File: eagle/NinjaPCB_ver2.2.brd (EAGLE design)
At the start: 79 x 73 mm, 72 parts, among them IC1 ANALOGSW_AD_SOT23-6, IC2 NAU7802, Q1 IRLB3813PBF, Q2 CJ2302, Q3 CJ2302, Q4 S9013, Q5 S9013, Q6 S9013

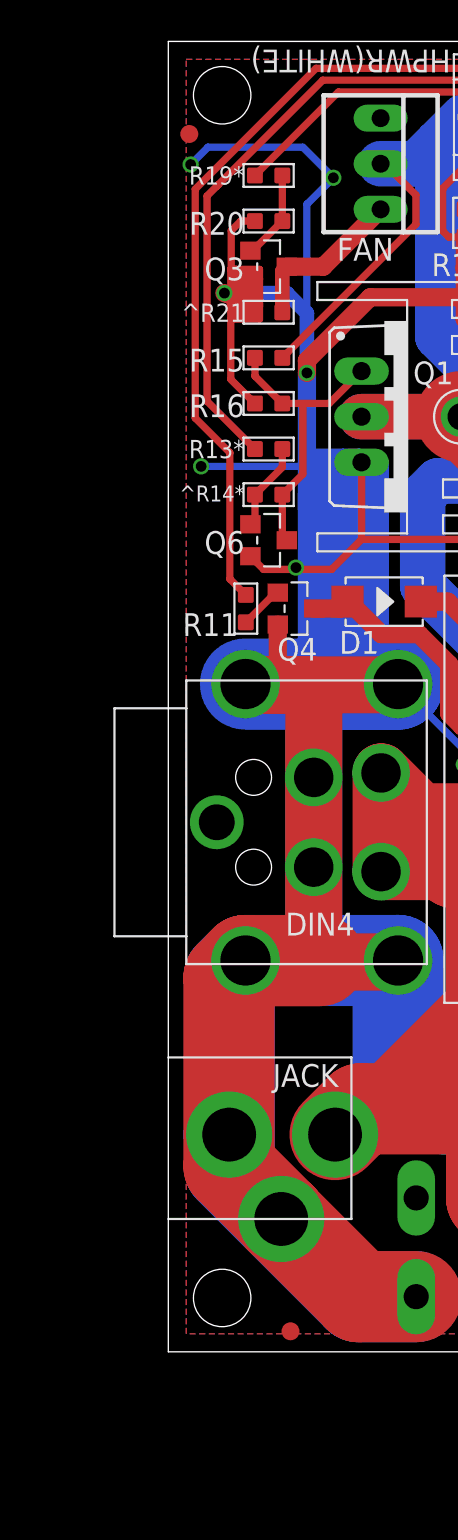
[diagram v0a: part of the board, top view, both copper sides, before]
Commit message: sync
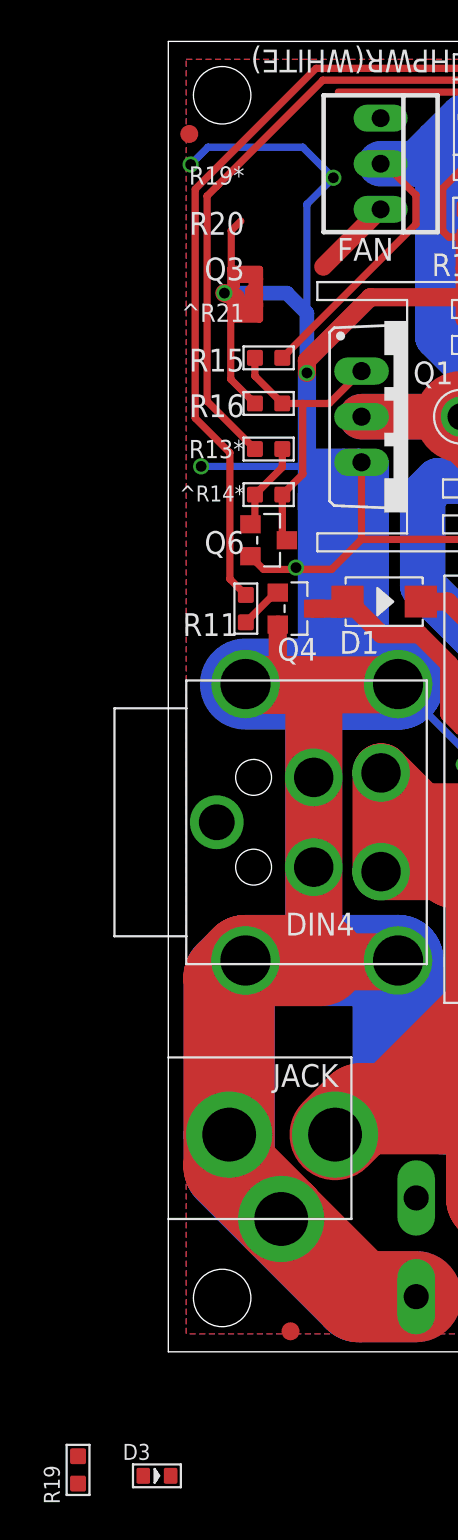
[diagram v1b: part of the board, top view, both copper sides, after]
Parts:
- removed Q3: CJ2302, Seeed-Transistor:SOT-23
- removed R20: 10K 1/10W, Seeed-Resistor:R0603
- removed R21: 0R, Seeed-Resistor:R0603
- added D3: YELLOW-0603, Seeed-LED:LED-0603
- R14: value 1K 1/10W -> 0R
- moved R19 72.9 mm to (-5.03, -6.58), turned to 0 degrees
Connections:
- net MODE renamed TOUT
- removed net FAN: ESP1.18, ESP2.P$8, ESP3.P$8, IO0.1, R19.1, R2.2
- removed net N$8: Q3.1, R19.2, R20.2
- new net IO0: D3.+, ESP1.18, ESP2.P$8, ESP3.P$8, IO0.1, R2.2
- net GND: now also FAN.3, R19.1; no longer Q3.2, R20.1, R21.1
- net N$4: now also D3.-, R19.2; no longer FAN.3, Q3.3, R21.2
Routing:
- net FAN: track 165.0 -> 0.00 mm, vias 3 -> 0
- net IO0: track 0.00 -> 158.4 mm, vias 0 -> 3
- net N$4: track 9.19 -> 0.00 mm
- net N$8: track 5.00 -> 0.00 mm
- net GND: track 878.0 -> 879.6 mm
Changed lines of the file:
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@@
 <attribute name="MPN" value="RC0603JR-0710KL" x="138.176" y="130.1496" size="1.778" layer="27" rot="R90" display="off"/>
-</element>
-<element name="R19" library="Seeed-Resistor" package="R0603" value="1K 1/10W" x="5.588" y="65.532" smashed="yes" rot="R90">
-<attribute name="MPN" value="RC0603JR-071KL" x="102.108" y="146.812" size="1.778" layer="27" rot="R90" display="off"/>
 </element>
 <element name="R17" library="Seeed-Resistor" package="R0603" value="1K 1/10W" x="19.05" y="62.8904" smashed="yes">
@@
 <element name="R18" library="Seeed-Resistor" package="R0603" value="10K 1/10W" x="16.51" y="62.8904" smashed="yes" rot="R180">
 <attribute name="MPN" value="RC0603JR-0710KL" x="-34.29" y="159.4104" size="1.778" layer="27" rot="R180" display="off"/>
-</element>
-<element name="R20" library="Seeed-Resistor" package="R0603" value="10K 1/10W" x="5.588" y="62.992" smashed="yes" rot="R90">
-<attribute name="MPN" value="RC0603JR-0710KL" x="102.108" y="118.872" size="1.778" layer="27" rot="R90" display="off"/>
 </element>
 <element name="R13" library="Seeed-Resistor" package="R0603" value="1K 1/10W" x="5.588" y="50.292" smashed="yes" rot="R90">
@@
 <element name="Q2" library="Seeed-Transistor" package="SOT-23" value="CJ2302" x="26.0434" y="59.635" smashed="yes" rot="R270">
 <attribute name="MPN" value="CJ2302" x="-55.2366" y="-1.325" size="1.778" layer="27" rot="R270" display="off"/>
-</element>
-<element name="Q3" library="Seeed-Transistor" package="SOT-23" value="CJ2302" x="5.588" y="60.452" smashed="yes" rot="R270">
-<attribute name="MPN" value="CJ2302" x="-75.692" y="-5.588" size="1.778" layer="27" rot="R270" display="off"/>
 </element>
 <element name="SERIAL6" library="pinhead" package="1X06" value="" x="45.0342" y="13.1826" smashed="yes" rot="MR0">
@@
 <element name="U$9" library="adafruit" package="FIDUCIAL_1MM" value="FIDUCIAL" x="53.467" y="46.609" smashed="yes" rot="R270"/>
 <element name="U$10" library="adafruit" package="FIDUCIAL_1MM" value="FIDUCIAL" x="77.851" y="40.513" smashed="yes" rot="R270"/>
-<element name="R14" library="Seeed-Resistor" package="R0603" value="1K 1/10W" x="5.588" y="47.752" smashed="yes" rot="R90">
-<attribute name="MPN" value="RC0603JR-071KL" x="102.108" y="134.112" size="1.778" layer="27" rot="R90" display="off"/>
-</element>
-<element name="R21" library="Seeed-Resistor" package="R0603" value="0R" x="5.588" y="57.912" smashed="yes" rot="R90">
-<attribute name="MPN" value="RC0603JR-070RL" x="108.458" y="117.602" size="1.778" layer="27" rot="R90" display="off"/>
+<element name="R14" library="Seeed-Resistor" package="R0603" value="0R" x="5.588" y="47.752" smashed="yes" rot="R90">
+<attribute name="MPN" value="RC0603JR-070RL" x="102.108" y="134.112" size="1.778" layer="27" rot="R90" display="off"/>
 </element>
 <element name="PELTIER" library="Seeed-Connector" package="H2-3.5-7.0X7.0MM" value="" x="35.775" y="34.9708" smashed="yes">
@@
 <element name="U$1" library="oshw" package="OSHW_5MM" value="" x="68.834" y="69.5198"/>
 <element name="U$2" library="oshw" package="OSHW_5MM" value="" x="75.3872" y="64.5922" rot="MR0"/>
+<element name="D3" library="Seeed-LED" package="LED-0603" value="YELLOW-0603" x="-0.635" y="-6.9088">
+<attribute name="MPN" value="19-217-Y5C-AM1N1VY-3T" x="-0.635" y="-6.9088" size="1.778" layer="27" display="off"/>
+</element>
+<element name="R19" library="Seeed-Resistor" package="R0603" value="1K 1/10W" x="-5.0292" y="-6.5786">
+<attribute name="MPN" value="RC0603JR-071KL" x="-5.0292" y="-6.5786" size="1.778" layer="27" display="off"/>
+</element>
 </elements>
 <signals>
@@
 <contactref element="Q2" pad="2"/>
 <contactref element="R18" pad="1"/>
-<contactref element="Q3" pad="2"/>
-<contactref element="R20" pad="1"/>
-<contactref element="R21" pad="1"/>
 <contactref element="SERIAL6" pad="6"/>
 <contactref element="ESP3" pad="P$9"/>
@@
 <wire x1="9.0932" y1="43.5864" x2="10.7638" y2="45.257" width="0.4064" layer="1"/>
 <wire x1="10.7638" y1="45.257" x2="10.7638" y2="49.5542" width="0.4064" layer="1"/>
-<wire x1="4.826" y1="59.309" x2="4.572" y2="59.563" width="0.4064" layer="1"/>
-<wire x1="4.826" y1="62.992" x2="4.0386" y2="62.992" width="0.4064" layer="1"/>
 <via x="3.1242" y="58.9788" extent="1-16" drill="0.6" shape="square"/>
 <wire x1="3.1242" y1="58.9788" x2="3.7592" y2="58.7502" width="1.016" layer="1"/>
-<wire x1="3.7592" y1="58.7502" x2="4.572" y2="59.563" width="1.016" layer="1"/>
-<wire x1="4.2926" y1="59.563" x2="4.572" y2="59.563" width="0.4064" layer="1"/>
 <wire x1="4.7752" y1="57.8866" x2="3.9624" y2="57.8866" width="0.8128" layer="1"/>
 <wire x1="3.9624" y1="57.8866" x2="3.6576" y2="58.1914" width="0.8128" layer="1"/>
@@
 <wire x1="3.5052" y1="60.325" x2="4.064" y2="59.7662" width="0.4064" layer="1"/>
 <wire x1="4.064" y1="59.7662" x2="4.3688" y2="59.7662" width="0.4064" layer="1"/>
-<wire x1="4.3688" y1="59.7662" x2="4.572" y2="59.563" width="0.4064" layer="1"/>
-<wire x1="4.826" y1="57.912" x2="4.8006" y2="57.912" width="0.4064" layer="1"/>
 <wire x1="4.8006" y1="57.912" x2="4.7752" y2="57.8866" width="0.4064" layer="1"/>
 <wire x1="8.4836" y1="49.2252" x2="10.4348" y2="49.2252" width="1.016" layer="16"/>
@@
 <wire x1="51.3588" y1="53.6702" x2="50.5206" y2="52.832" width="0.4064" layer="1"/>
 <wire x1="50.5206" y1="52.832" x2="48.768" y2="52.832" width="0.4064" layer="1"/>
+<contactref element="FAN" pad="3"/>
+<wire x1="11.8274" y1="63.6456" x2="8.6338" y2="60.452" width="1.016" layer="1"/>
+<contactref element="R19" pad="1"/>
+<wire x1="56.7436" y1="25.2984" x2="51.7398" y2="29.4386" width="0" layer="19" extent="1-1"/>
+<wire x1="5.08" y1="59.7408" x2="4.8768" y2="59.817" width="0" layer="19" extent="1-1"/>
+<wire x1="8.6338" y1="60.452" x2="6.604" y2="58.9788" width="0" layer="19" extent="1-16"/>
+<wire x1="71.7804" y1="3.2004" x2="77.159" y2="6.817" width="0" layer="19" extent="1-1"/>
+<wire x1="61.7982" y1="5.8674" x2="67.6656" y2="11.1252" width="0" layer="19" extent="1-1"/>
+<wire x1="-5.0292" y1="-5.8166" x2="6.29" y2="7.4" width="0" layer="19" extent="1-1"/>
 </signal>
 <signal name="3V3">
@@
 <wire x1="32.893" y1="47.4472" x2="33.0454" y2="47.4472" width="0.4064" layer="16"/>
 </signal>
-<signal name="N$4">
-<contactref element="FAN" pad="3"/>
-<contactref element="Q3" pad="3"/>
-<contactref element="R21" pad="2"/>
-<wire x1="11.8274" y1="63.6456" x2="8.6338" y2="60.452" width="1.016" layer="1"/>
-<wire x1="8.6338" y1="60.452" x2="6.604" y2="60.452" width="1.016" layer="1"/>
-<wire x1="6.35" y1="57.912" x2="6.35" y2="60.198" width="0.8128" layer="1"/>
-<wire x1="6.35" y1="60.198" x2="6.604" y2="60.452" width="0.8128" layer="1"/>
-</signal>
-<signal name="FAN">
-<contactref element="R19" pad="1"/>
+<signal name="IO0">
 <contactref element="ESP2" pad="P$8"/>
 <contactref element="ESP1" pad="18"/>
@@
 <contactref element="ESP3" pad="P$8"/>
 <contactref element="IO0" pad="1"/>
-<wire x1="4.826" y1="65.532" x2="9.4742" y2="70.1802" width="0.4064" layer="1"/>
 <wire x1="58.1844" y1="43.239" x2="58.1844" y2="41.6884" width="0.4064" layer="1"/>
 <wire x1="58.1844" y1="41.6884" x2="58.9026" y2="40.9702" width="0.4064" layer="1"/>
@@
 <wire x1="60.7568" y1="52.9336" x2="59.1312" y2="54.5592" width="0.4064" layer="1"/>
 <wire x1="59.1312" y1="54.5592" x2="59.1312" y2="59.5884" width="0.4064" layer="1"/>
+<contactref element="D3" pad="+"/>
+<wire x1="-1.397" y1="-6.9088" x2="42.4942" y2="11.6586" width="0" layer="19" extent="1-1"/>
 </signal>
 <signal name="PEL_PWM">
@@
 <wire x1="32.512" y1="61.976" x2="32.512" y2="62.992" width="0.4064" layer="1"/>
 </signal>
-<signal name="MODE">
+<signal name="TOUT">
 <contactref element="ESP1" pad="2"/>
 <contactref element="ESP2" pad="P$16"/>
@@
 <wire x1="65.405" y1="58.166" x2="65.7352" y2="57.8358" width="0.4064" layer="16"/>
 </signal>
-<signal name="N$8">
+<signal name="N$4">
+<contactref element="D3" pad="-"/>
 <contactref element="R19" pad="2"/>
-<contactref element="Q3" pad="1"/>
-<contactref element="R20" pad="2"/>
-<wire x1="4.572" y1="61.341" x2="4.699" y2="61.341" width="0.4064" layer="1"/>
-<wire x1="4.699" y1="61.341" x2="6.35" y2="62.992" width="0.4064" layer="1"/>
-<wire x1="6.35" y1="65.532" x2="6.35" y2="62.992" width="0.4064" layer="1"/>
+<wire x1="0.127" y1="-6.9088" x2="-5.0292" y2="-7.3406" width="0" layer="19" extent="1-1"/>
 </signal>
 </signals>

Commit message: add NinjaPCR 2.2
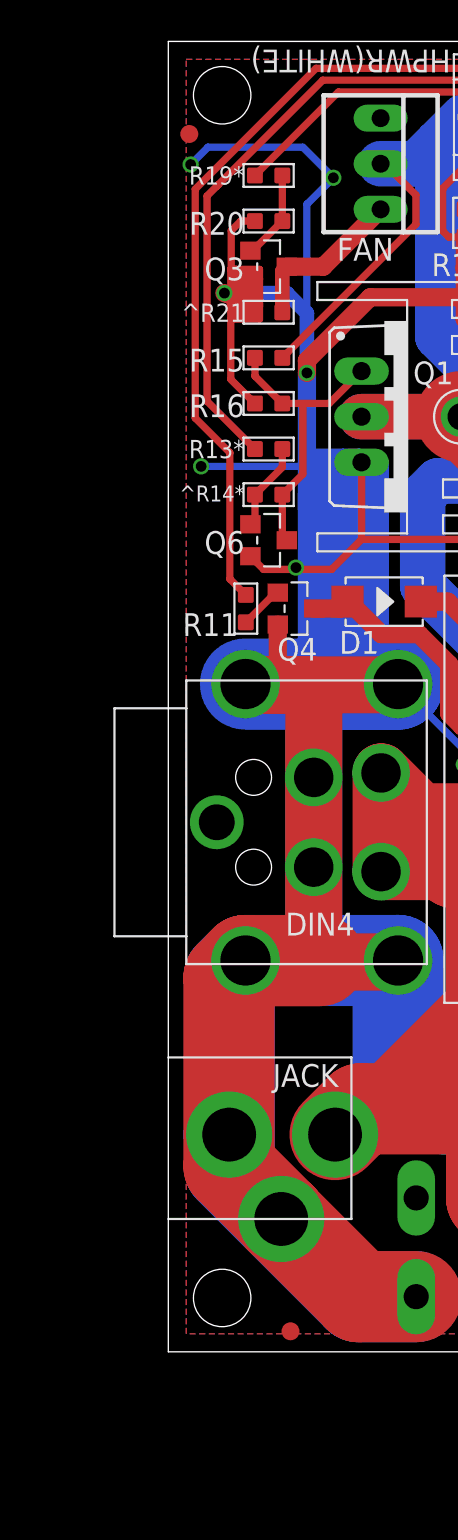
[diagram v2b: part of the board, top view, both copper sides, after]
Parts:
- removed D3: YELLOW-0603, Seeed-LED:LED-0603
- added Q3: CJ2302, Seeed-Transistor:SOT-23
- added R20: 10K 1/10W, Seeed-Resistor:R0603
- added R21: 0R, Seeed-Resistor:R0603
- R14: value 0R -> 1K 1/10W
- moved R19 72.9 mm to (5.59, 65.5), turned to 90 degrees
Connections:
- net TOUT renamed MODE
- removed net IO0: D3.+, ESP1.18, ESP2.P$8, ESP3.P$8, IO0.1, R2.2
- new net FAN: ESP1.18, ESP2.P$8, ESP3.P$8, IO0.1, R19.1, R2.2
- new net N$8: Q3.1, R19.2, R20.2
- net GND: now also Q3.2, R20.1, R21.1; no longer FAN.3, R19.1
- net N$4: now also FAN.3, Q3.3, R21.2; no longer D3.-, R19.2
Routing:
- net FAN: track 0.00 -> 165.0 mm, vias 0 -> 3
- net IO0: track 158.4 -> 0.00 mm, vias 3 -> 0
- net N$4: track 0.00 -> 9.19 mm
- net N$8: track 0.00 -> 5.00 mm
- net GND: track 879.6 -> 878.0 mm
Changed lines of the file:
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@@
 <attribute name="MPN" value="RC0603JR-0710KL" x="138.176" y="130.1496" size="1.778" layer="27" rot="R90" display="off"/>
+</element>
+<element name="R19" library="Seeed-Resistor" package="R0603" value="1K 1/10W" x="5.588" y="65.532" smashed="yes" rot="R90">
+<attribute name="MPN" value="RC0603JR-071KL" x="102.108" y="146.812" size="1.778" layer="27" rot="R90" display="off"/>
 </element>
 <element name="R17" library="Seeed-Resistor" package="R0603" value="1K 1/10W" x="19.05" y="62.8904" smashed="yes">
@@
 <element name="R18" library="Seeed-Resistor" package="R0603" value="10K 1/10W" x="16.51" y="62.8904" smashed="yes" rot="R180">
 <attribute name="MPN" value="RC0603JR-0710KL" x="-34.29" y="159.4104" size="1.778" layer="27" rot="R180" display="off"/>
+</element>
+<element name="R20" library="Seeed-Resistor" package="R0603" value="10K 1/10W" x="5.588" y="62.992" smashed="yes" rot="R90">
+<attribute name="MPN" value="RC0603JR-0710KL" x="102.108" y="118.872" size="1.778" layer="27" rot="R90" display="off"/>
 </element>
 <element name="R13" library="Seeed-Resistor" package="R0603" value="1K 1/10W" x="5.588" y="50.292" smashed="yes" rot="R90">
@@
 <element name="Q2" library="Seeed-Transistor" package="SOT-23" value="CJ2302" x="26.0434" y="59.635" smashed="yes" rot="R270">
 <attribute name="MPN" value="CJ2302" x="-55.2366" y="-1.325" size="1.778" layer="27" rot="R270" display="off"/>
+</element>
+<element name="Q3" library="Seeed-Transistor" package="SOT-23" value="CJ2302" x="5.588" y="60.452" smashed="yes" rot="R270">
+<attribute name="MPN" value="CJ2302" x="-75.692" y="-5.588" size="1.778" layer="27" rot="R270" display="off"/>
 </element>
 <element name="SERIAL6" library="pinhead" package="1X06" value="" x="45.0342" y="13.1826" smashed="yes" rot="MR0">
@@
 <element name="U$9" library="adafruit" package="FIDUCIAL_1MM" value="FIDUCIAL" x="53.467" y="46.609" smashed="yes" rot="R270"/>
 <element name="U$10" library="adafruit" package="FIDUCIAL_1MM" value="FIDUCIAL" x="77.851" y="40.513" smashed="yes" rot="R270"/>
-<element name="R14" library="Seeed-Resistor" package="R0603" value="0R" x="5.588" y="47.752" smashed="yes" rot="R90">
-<attribute name="MPN" value="RC0603JR-070RL" x="102.108" y="134.112" size="1.778" layer="27" rot="R90" display="off"/>
+<element name="R14" library="Seeed-Resistor" package="R0603" value="1K 1/10W" x="5.588" y="47.752" smashed="yes" rot="R90">
+<attribute name="MPN" value="RC0603JR-071KL" x="102.108" y="134.112" size="1.778" layer="27" rot="R90" display="off"/>
+</element>
+<element name="R21" library="Seeed-Resistor" package="R0603" value="0R" x="5.588" y="57.912" smashed="yes" rot="R90">
+<attribute name="MPN" value="RC0603JR-070RL" x="108.458" y="117.602" size="1.778" layer="27" rot="R90" display="off"/>
 </element>
 <element name="PELTIER" library="Seeed-Connector" package="H2-3.5-7.0X7.0MM" value="" x="35.775" y="34.9708" smashed="yes">
@@
 <element name="U$1" library="oshw" package="OSHW_5MM" value="" x="68.834" y="69.5198"/>
 <element name="U$2" library="oshw" package="OSHW_5MM" value="" x="75.3872" y="64.5922" rot="MR0"/>
-<element name="D3" library="Seeed-LED" package="LED-0603" value="YELLOW-0603" x="-0.635" y="-6.9088">
-<attribute name="MPN" value="19-217-Y5C-AM1N1VY-3T" x="-0.635" y="-6.9088" size="1.778" layer="27" display="off"/>
-</element>
-<element name="R19" library="Seeed-Resistor" package="R0603" value="1K 1/10W" x="-5.0292" y="-6.5786">
-<attribute name="MPN" value="RC0603JR-071KL" x="-5.0292" y="-6.5786" size="1.778" layer="27" display="off"/>
-</element>
 </elements>
 <signals>
@@
 <contactref element="Q2" pad="2"/>
 <contactref element="R18" pad="1"/>
+<contactref element="Q3" pad="2"/>
+<contactref element="R20" pad="1"/>
+<contactref element="R21" pad="1"/>
 <contactref element="SERIAL6" pad="6"/>
 <contactref element="ESP3" pad="P$9"/>
@@
 <wire x1="9.0932" y1="43.5864" x2="10.7638" y2="45.257" width="0.4064" layer="1"/>
 <wire x1="10.7638" y1="45.257" x2="10.7638" y2="49.5542" width="0.4064" layer="1"/>
+<wire x1="4.826" y1="59.309" x2="4.572" y2="59.563" width="0.4064" layer="1"/>
+<wire x1="4.826" y1="62.992" x2="4.0386" y2="62.992" width="0.4064" layer="1"/>
 <via x="3.1242" y="58.9788" extent="1-16" drill="0.6" shape="square"/>
 <wire x1="3.1242" y1="58.9788" x2="3.7592" y2="58.7502" width="1.016" layer="1"/>
+<wire x1="3.7592" y1="58.7502" x2="4.572" y2="59.563" width="1.016" layer="1"/>
+<wire x1="4.2926" y1="59.563" x2="4.572" y2="59.563" width="0.4064" layer="1"/>
 <wire x1="4.7752" y1="57.8866" x2="3.9624" y2="57.8866" width="0.8128" layer="1"/>
 <wire x1="3.9624" y1="57.8866" x2="3.6576" y2="58.1914" width="0.8128" layer="1"/>
@@
 <wire x1="3.5052" y1="60.325" x2="4.064" y2="59.7662" width="0.4064" layer="1"/>
 <wire x1="4.064" y1="59.7662" x2="4.3688" y2="59.7662" width="0.4064" layer="1"/>
+<wire x1="4.3688" y1="59.7662" x2="4.572" y2="59.563" width="0.4064" layer="1"/>
+<wire x1="4.826" y1="57.912" x2="4.8006" y2="57.912" width="0.4064" layer="1"/>
 <wire x1="4.8006" y1="57.912" x2="4.7752" y2="57.8866" width="0.4064" layer="1"/>
 <wire x1="8.4836" y1="49.2252" x2="10.4348" y2="49.2252" width="1.016" layer="16"/>
@@
 <wire x1="51.3588" y1="53.6702" x2="50.5206" y2="52.832" width="0.4064" layer="1"/>
 <wire x1="50.5206" y1="52.832" x2="48.768" y2="52.832" width="0.4064" layer="1"/>
-<contactref element="FAN" pad="3"/>
-<wire x1="11.8274" y1="63.6456" x2="8.6338" y2="60.452" width="1.016" layer="1"/>
-<contactref element="R19" pad="1"/>
-<wire x1="56.7436" y1="25.2984" x2="51.7398" y2="29.4386" width="0" layer="19" extent="1-1"/>
-<wire x1="5.08" y1="59.7408" x2="4.8768" y2="59.817" width="0" layer="19" extent="1-1"/>
-<wire x1="8.6338" y1="60.452" x2="6.604" y2="58.9788" width="0" layer="19" extent="1-16"/>
-<wire x1="71.7804" y1="3.2004" x2="77.159" y2="6.817" width="0" layer="19" extent="1-1"/>
-<wire x1="61.7982" y1="5.8674" x2="67.6656" y2="11.1252" width="0" layer="19" extent="1-1"/>
-<wire x1="-5.0292" y1="-5.8166" x2="6.29" y2="7.4" width="0" layer="19" extent="1-1"/>
 </signal>
 <signal name="3V3">
@@
 <wire x1="32.893" y1="47.4472" x2="33.0454" y2="47.4472" width="0.4064" layer="16"/>
 </signal>
-<signal name="IO0">
+<signal name="N$4">
+<contactref element="FAN" pad="3"/>
+<contactref element="Q3" pad="3"/>
+<contactref element="R21" pad="2"/>
+<wire x1="11.8274" y1="63.6456" x2="8.6338" y2="60.452" width="1.016" layer="1"/>
+<wire x1="8.6338" y1="60.452" x2="6.604" y2="60.452" width="1.016" layer="1"/>
+<wire x1="6.35" y1="57.912" x2="6.35" y2="60.198" width="0.8128" layer="1"/>
+<wire x1="6.35" y1="60.198" x2="6.604" y2="60.452" width="0.8128" layer="1"/>
+</signal>
+<signal name="FAN">
+<contactref element="R19" pad="1"/>
 <contactref element="ESP2" pad="P$8"/>
 <contactref element="ESP1" pad="18"/>
@@
 <contactref element="ESP3" pad="P$8"/>
 <contactref element="IO0" pad="1"/>
+<wire x1="4.826" y1="65.532" x2="9.4742" y2="70.1802" width="0.4064" layer="1"/>
 <wire x1="58.1844" y1="43.239" x2="58.1844" y2="41.6884" width="0.4064" layer="1"/>
 <wire x1="58.1844" y1="41.6884" x2="58.9026" y2="40.9702" width="0.4064" layer="1"/>
@@
 <wire x1="60.7568" y1="52.9336" x2="59.1312" y2="54.5592" width="0.4064" layer="1"/>
 <wire x1="59.1312" y1="54.5592" x2="59.1312" y2="59.5884" width="0.4064" layer="1"/>
-<contactref element="D3" pad="+"/>
-<wire x1="-1.397" y1="-6.9088" x2="42.4942" y2="11.6586" width="0" layer="19" extent="1-1"/>
 </signal>
 <signal name="PEL_PWM">
@@
 <wire x1="32.512" y1="61.976" x2="32.512" y2="62.992" width="0.4064" layer="1"/>
 </signal>
-<signal name="TOUT">
+<signal name="MODE">
 <contactref element="ESP1" pad="2"/>
 <contactref element="ESP2" pad="P$16"/>
@@
 <wire x1="65.405" y1="58.166" x2="65.7352" y2="57.8358" width="0.4064" layer="16"/>
 </signal>
-<signal name="N$4">
-<contactref element="D3" pad="-"/>
+<signal name="N$8">
 <contactref element="R19" pad="2"/>
-<wire x1="0.127" y1="-6.9088" x2="-5.0292" y2="-7.3406" width="0" layer="19" extent="1-1"/>
+<contactref element="Q3" pad="1"/>
+<contactref element="R20" pad="2"/>
+<wire x1="4.572" y1="61.341" x2="4.699" y2="61.341" width="0.4064" layer="1"/>
+<wire x1="4.699" y1="61.341" x2="6.35" y2="62.992" width="0.4064" layer="1"/>
+<wire x1="6.35" y1="65.532" x2="6.35" y2="62.992" width="0.4064" layer="1"/>
 </signal>
 </signals>
